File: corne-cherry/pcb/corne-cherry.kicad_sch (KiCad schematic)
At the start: 124 parts, among them J2 OLED, J3 MJ-4PP-9, J4 OLED, SW1 SW_PUSH, SW10 SW_PUSH, SW11 SW_PUSH, SW12 SW_PUSH, SW13 SW_PUSH, SW14 SW_PUSH, SW15 SW_PUSH, SW16 SW_PUSH, SW17 SW_PUSH, SW18 SW_PUSH, SW19 SW_PUSH, SW2 SW_PUSH, SW20 SW_PUSH, SW21 SW_PUSH, SW22 SW_PUSH, SW23 SW_PUSH, SW24 SW_PUSH, SW25 SW_PUSH, SW26 SW_PUSH, SW27 SW_PUSH, SW28 SW_PUSH, SW29 SW_PUSH, SW3 SW_PUSH, SW30 SW_PUSH, SW31 SW_PUSH, SW32 SW_PUSH, SW33 SW_PUSH, SW34 SW_PUSH, SW35 SW_PUSH, SW36 SW_PUSH, SW37 SW_PUSH, SW38 SW_PUSH, SW39 SW_PUSH, SW4 SW_PUSH, SW40 SW_PUSH, SW41 SW_PUSH, SW42 SW_PUSH, SW5 SW_PUSH, SW6 SW_PUSH, SW7 SW_PUSH, SW8 SW_PUSH, SW9 SW_PUSH, U1 ProMicro, U2 ProMicro

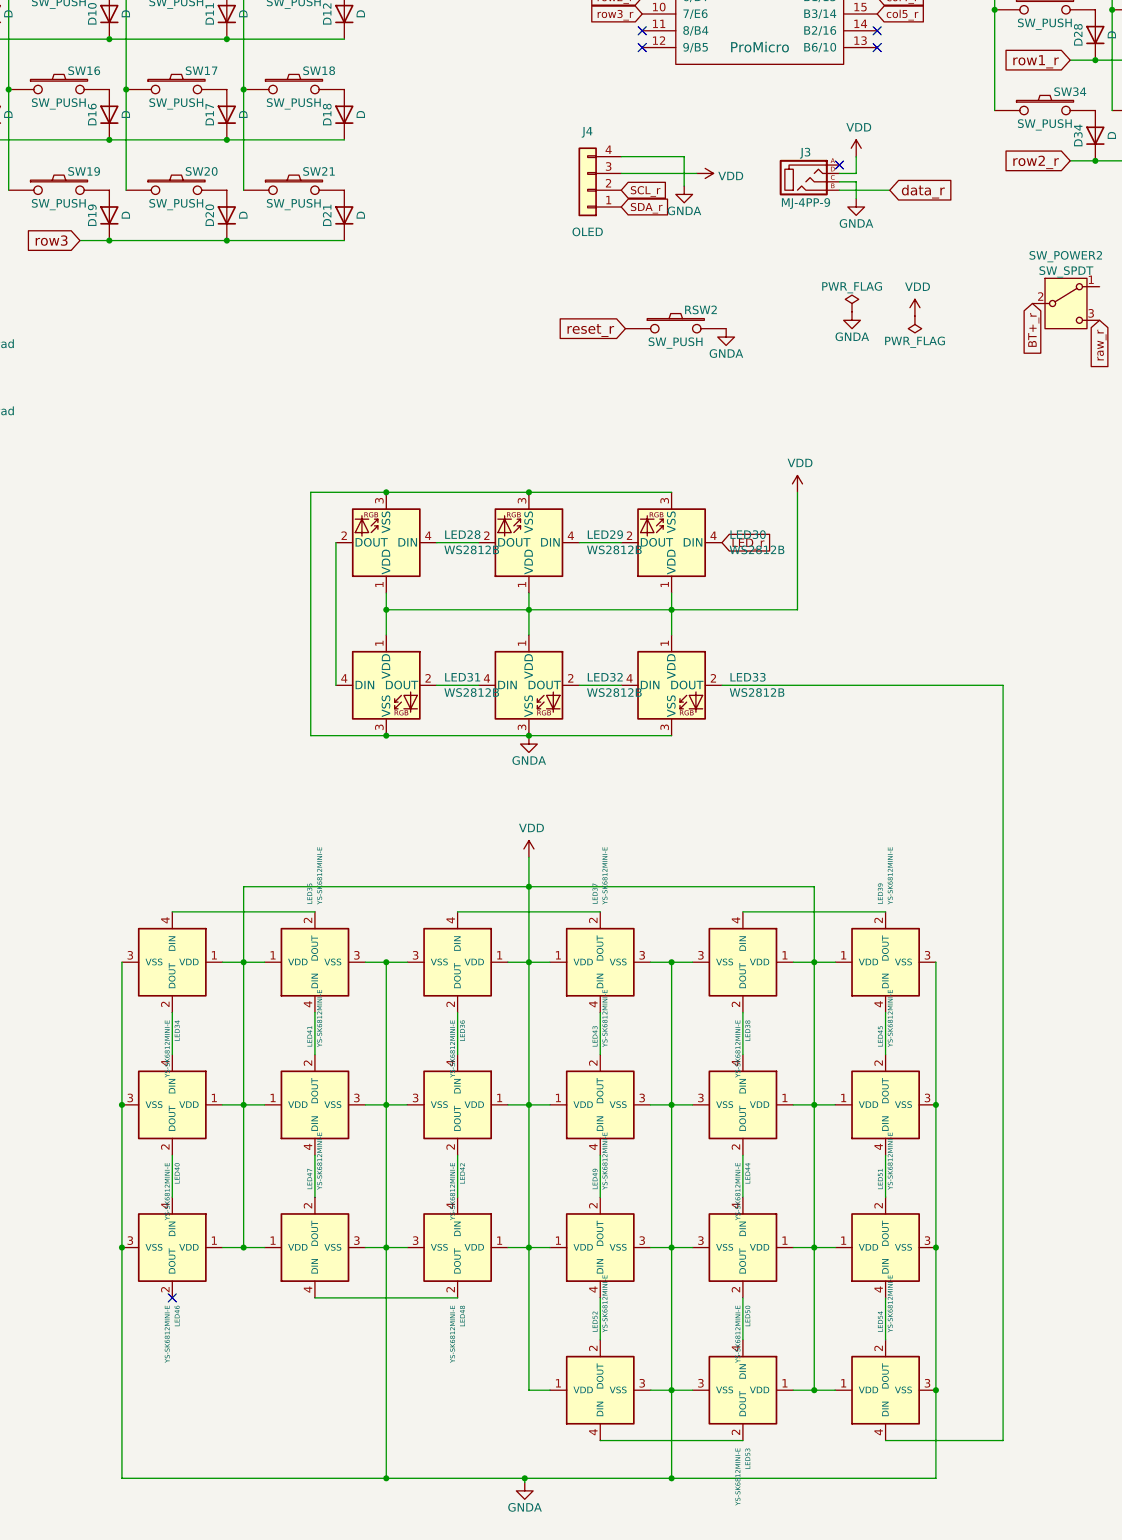
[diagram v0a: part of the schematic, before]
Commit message: finished all traces
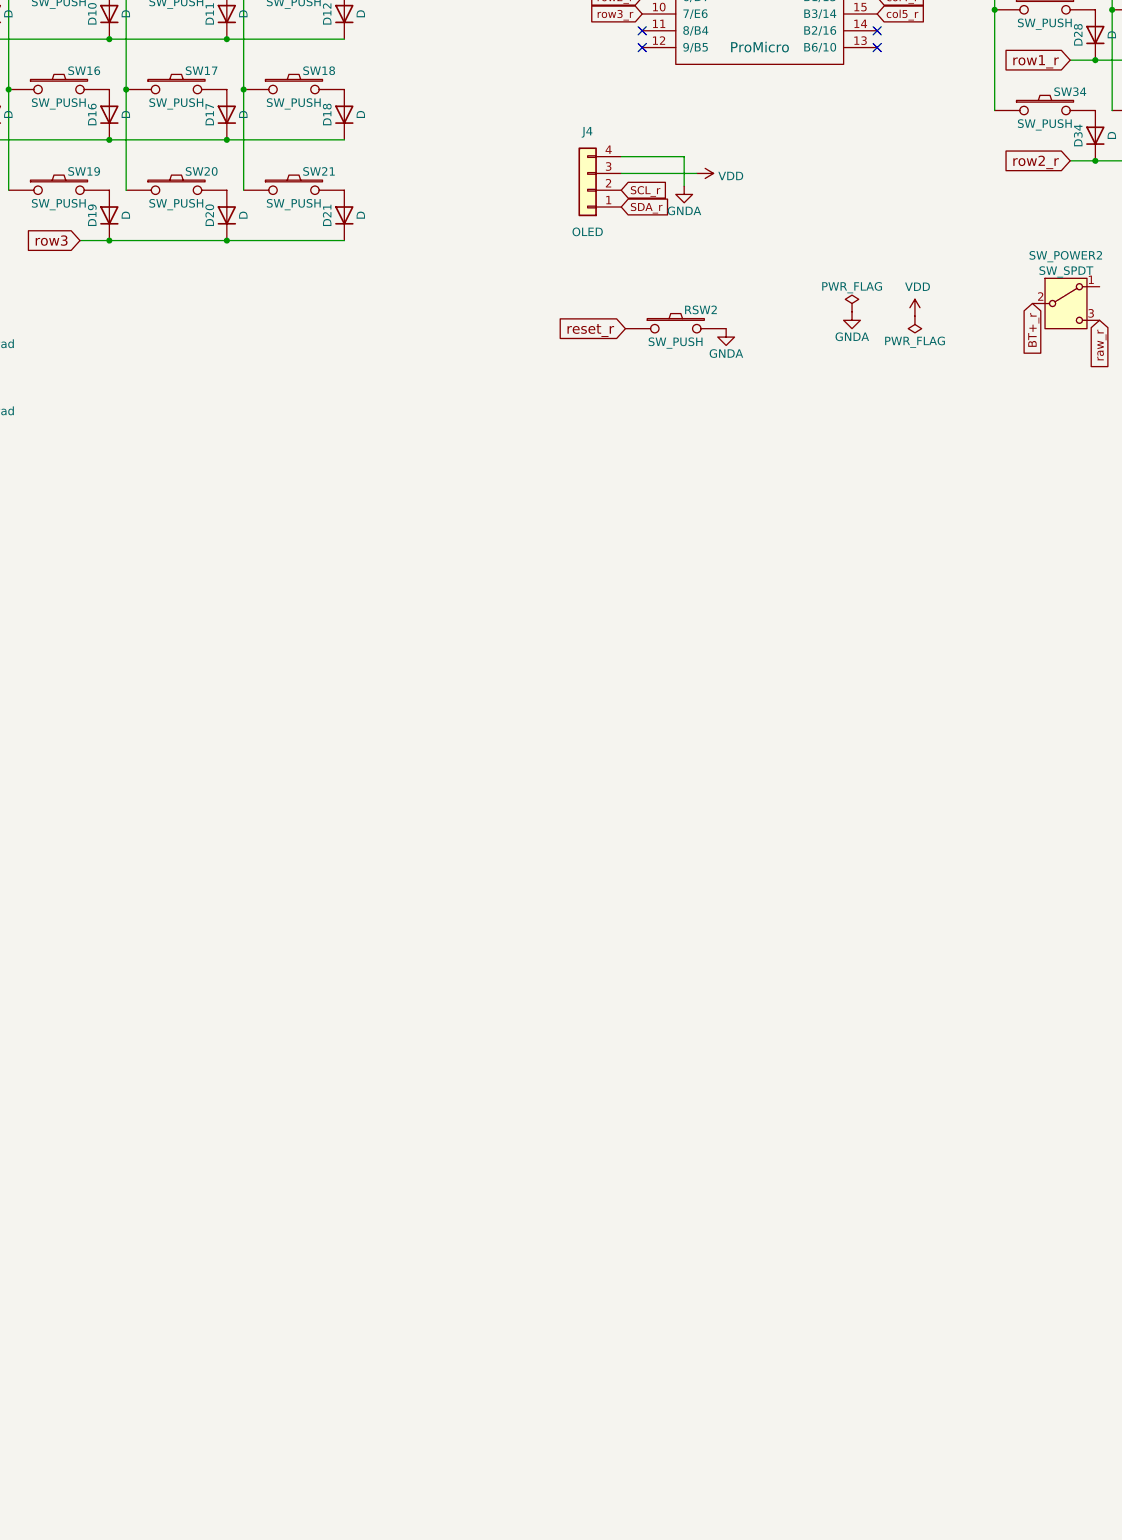
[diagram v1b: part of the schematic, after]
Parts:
- removed J3: MJ-4PP-9, kbd:MJ-4PP-9_1side, symbol kbd:MJ-4PP-9
- removed LED28, LED29, LED30, LED31, LED32, LED33: WS2812B, LED_SMD:LED_WS2812B_PLCC4_5.0x5.0mm_P3.2mm, symbol LED:WS2812B
- removed LED34, LED35, LED36, LED37, LED38, LED39, LED40, LED41, LED42, LED43, LED44, LED45, LED46, LED47, LED48, LED49, LED50, LED51, LED52, LED53, LED54: YS-SK6812MINI-E, kbd:YS-SK6812MINI-E, symbol kbd:YS-SK6812MINI-E
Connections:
- no-connect marks 10 -> 8
